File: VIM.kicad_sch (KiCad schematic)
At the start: 23 parts, among them U3 INA139, U4 MAX11615, U5 INA139

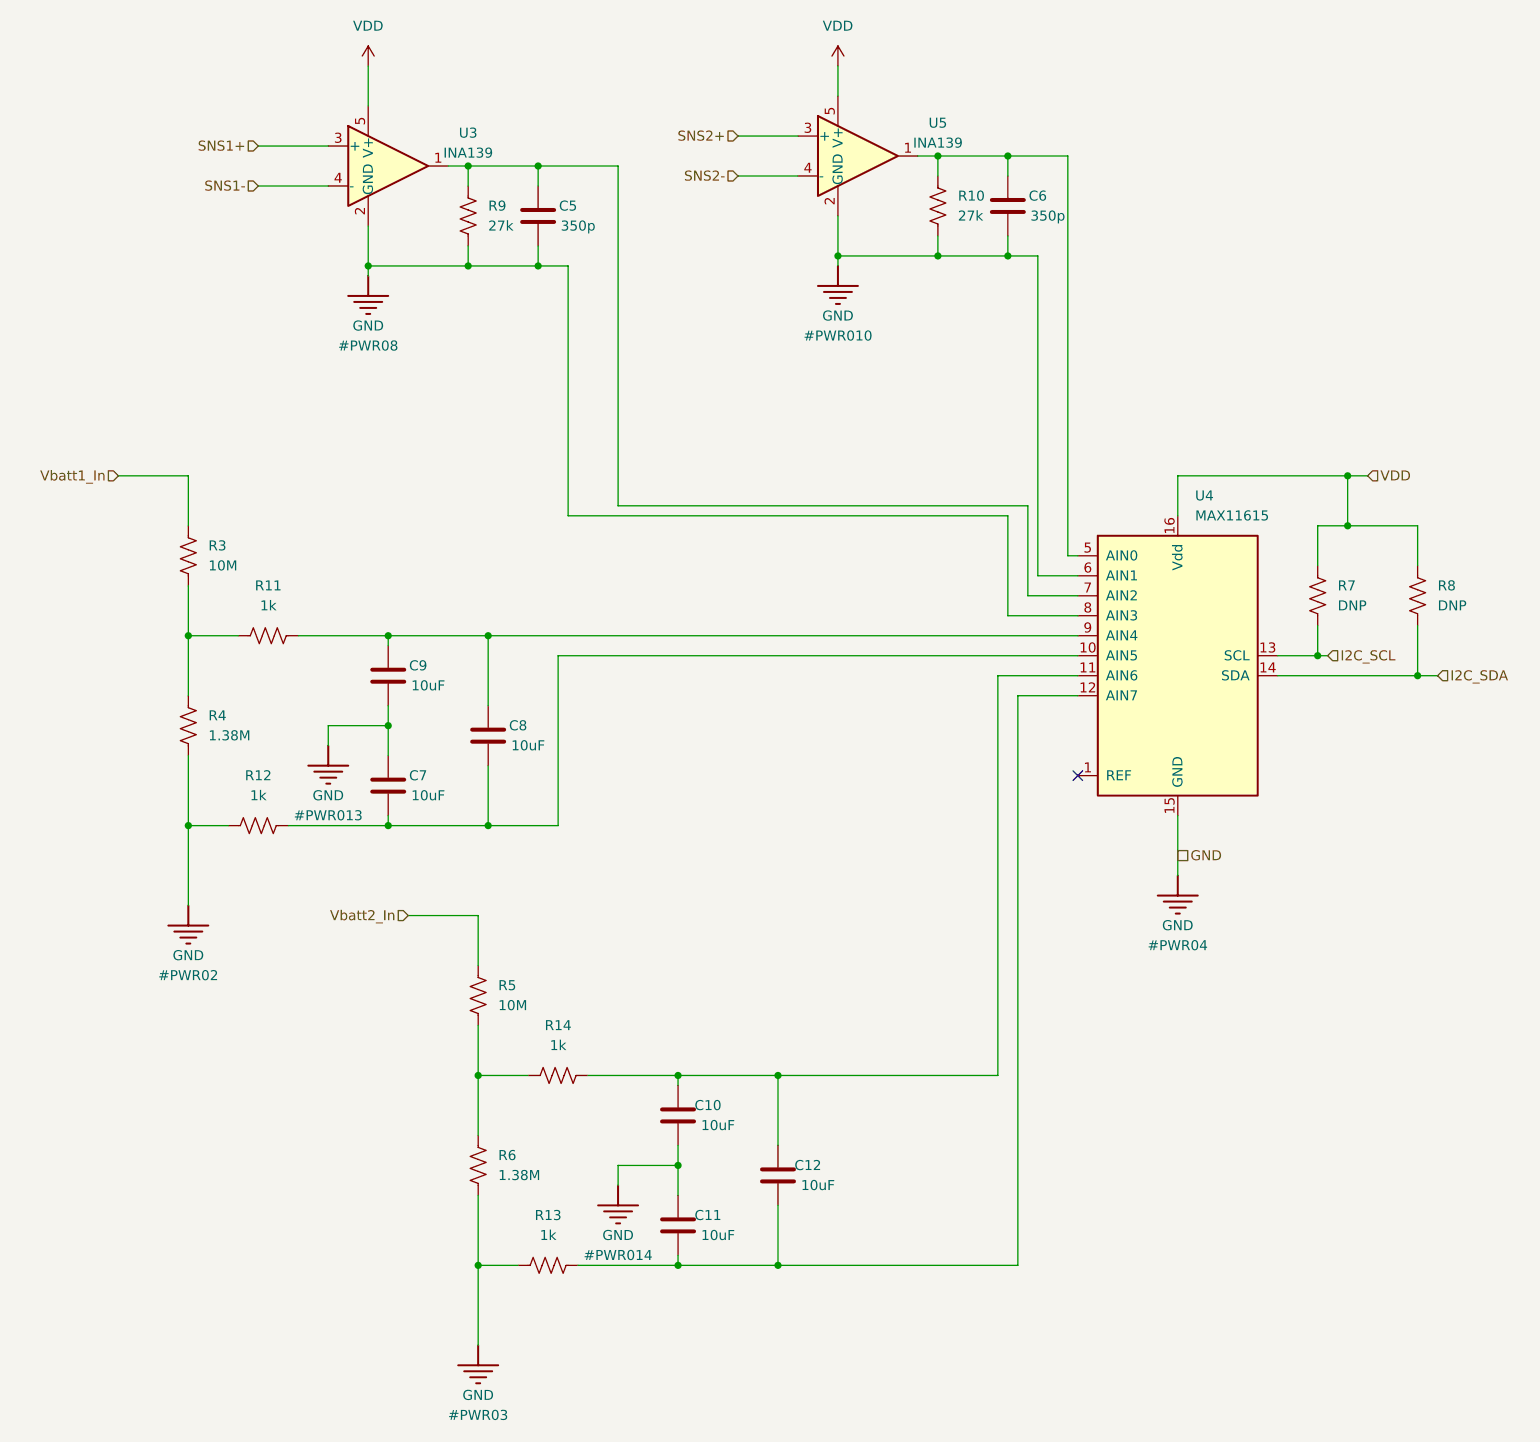
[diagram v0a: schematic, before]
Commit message: changed circuit
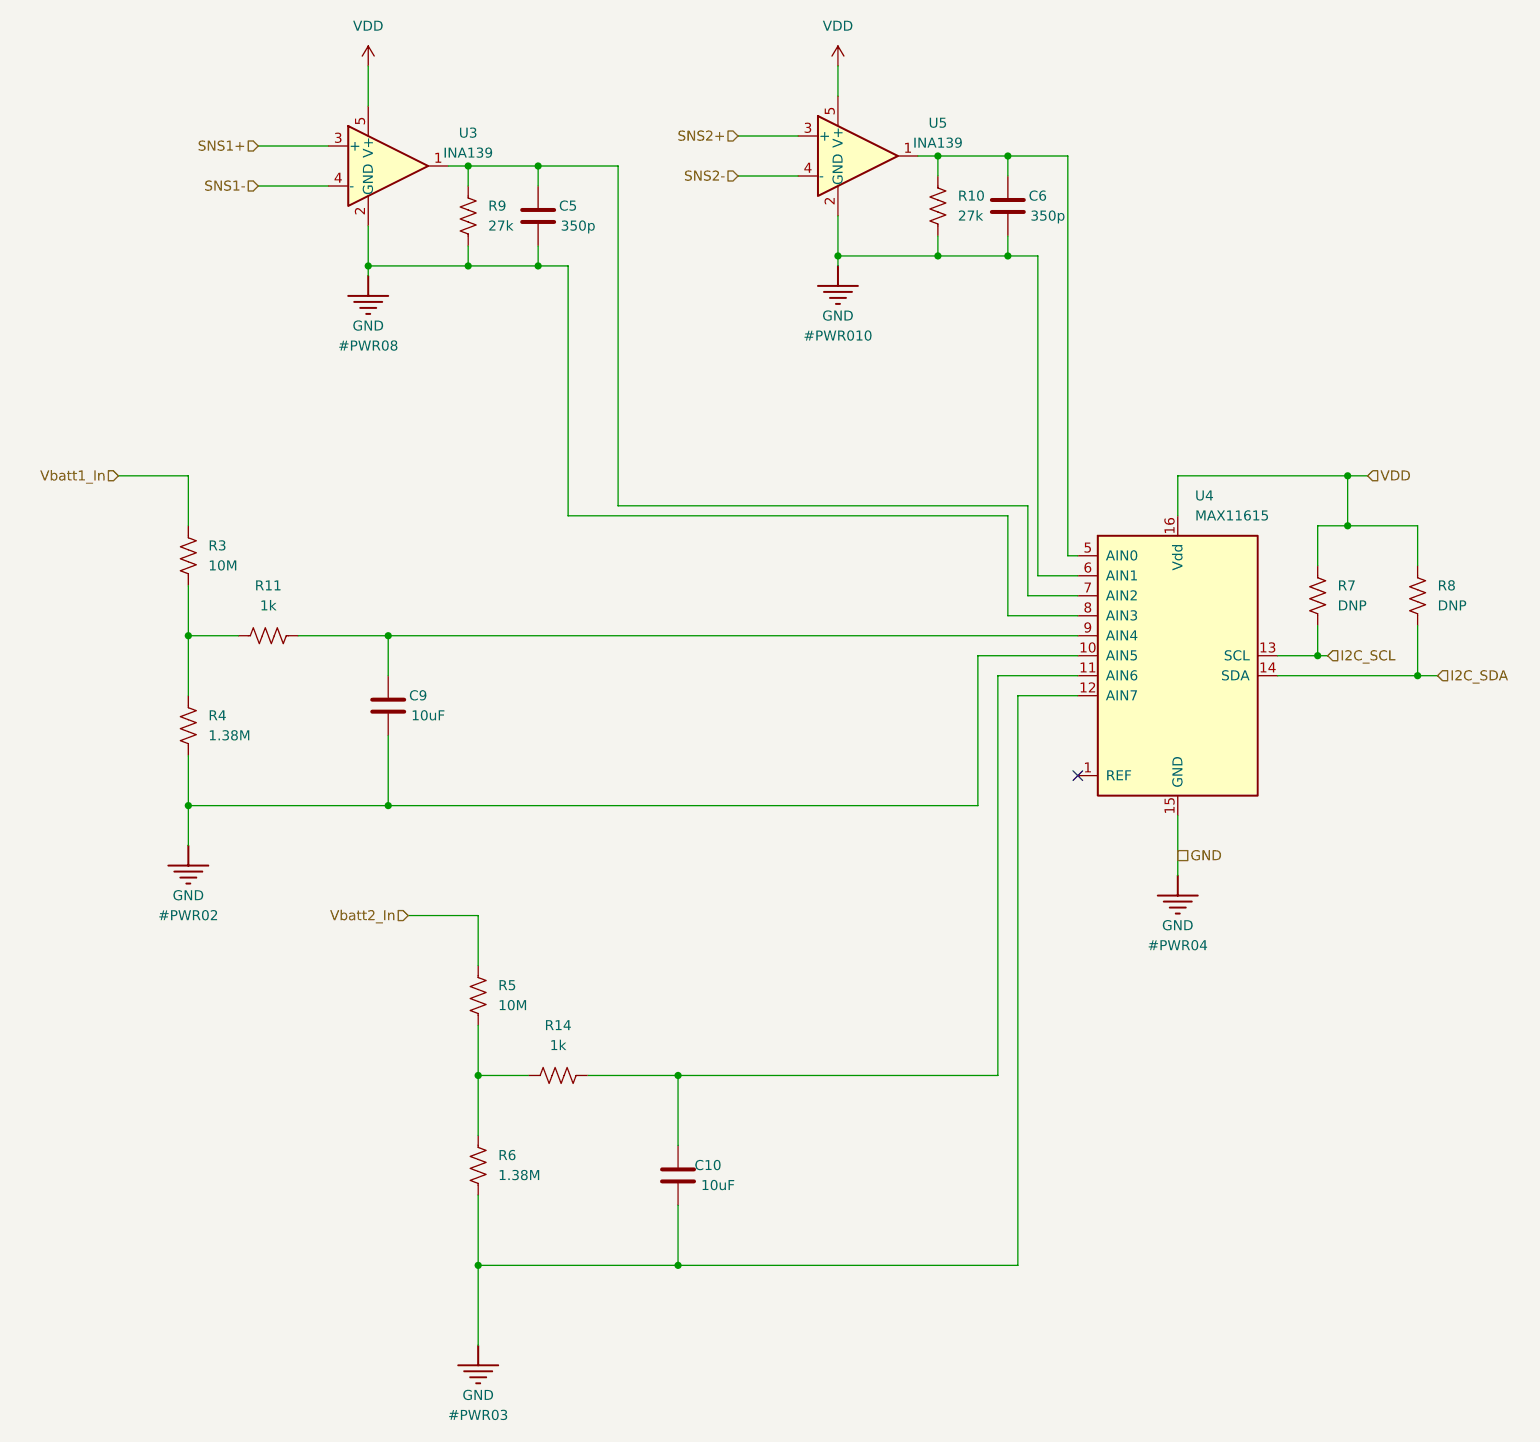
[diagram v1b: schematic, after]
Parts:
- removed C11, C12, C7, C8: 10uF, Capacitor_SMD:C_0805_2012Metric_Pad1.18x1.45mm_HandSolder, symbol Device:C
- removed R12, R13: 1k, Resistor_SMD:R_0805_2012Metric_Pad1.20x1.40mm_HandSolder, symbol Device:R_US
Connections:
- net GND: now also U4.10 (AIN5), U4.12 (AIN7)
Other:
- moved on the sheet: C10, C9
